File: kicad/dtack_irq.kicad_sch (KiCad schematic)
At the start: 18 parts, among them J10 Free pin, J11 Free Pins, J12 Free pins, J13 Free pins, J14 Free pin, J15 Free pin, J9 Free pin, U16 GAL22V10, U17 GAL22V10

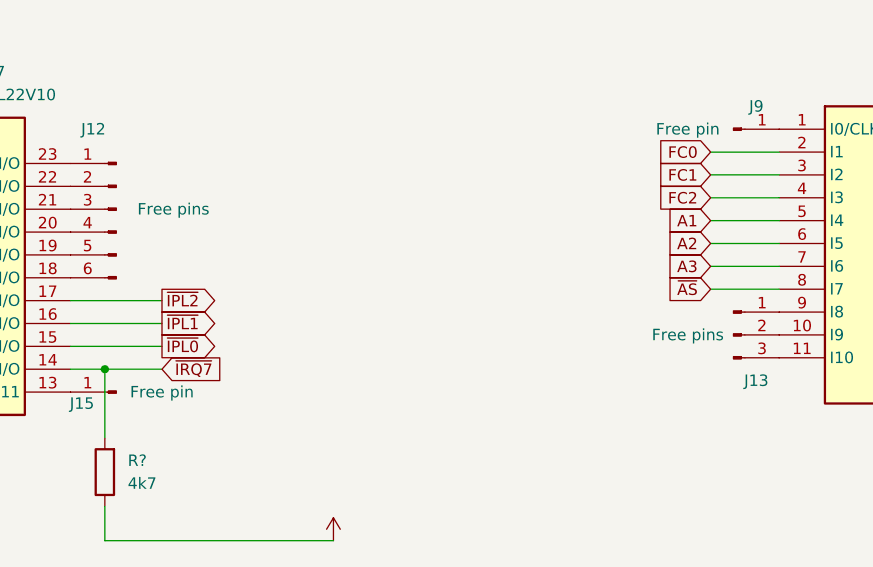
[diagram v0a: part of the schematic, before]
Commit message: fiddlign with placement
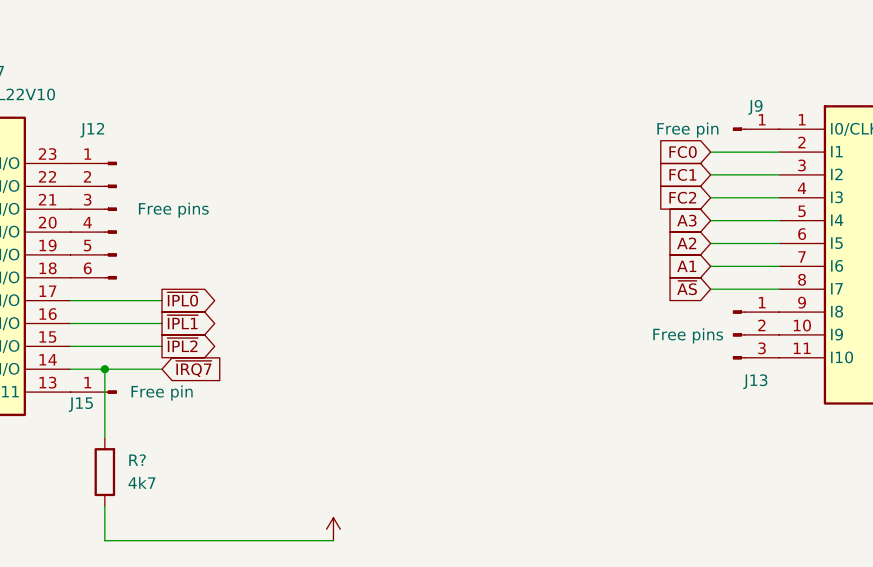
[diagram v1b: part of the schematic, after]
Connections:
- net A1: now also U16.7 (I6); no longer U16.5 (I4)
- net A3: now also U16.5 (I4); no longer U16.7 (I6)
- net ~{IPL0}: now also U17.17 (I/O); no longer U17.15 (I/O)
- net ~{IPL2}: now also U17.15 (I/O); no longer U17.17 (I/O)
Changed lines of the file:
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@@
     (effects (font (size 1.27 1.27)) (justify left bottom))
   )
-  (global_label "~{IPL2}" (shape output) (at 119.38 68.58 0) (fields_autoplaced)
+  (global_label "~{IPL2}" (shape output) (at 119.38 73.66 0) (fields_autoplaced)
     (effects (font (size 1.27 1.27)) (justify left))
-    (property "Intersheetrefs" "${INTERSHEET_REFS}" (at 126.3982 68.58 0)
+    (property "Intersheetrefs" "${INTERSHEET_REFS}" (at 126.3982 73.66 0)
       (effects (font (size 1.27 1.27)) (justify left) hide)
     )
@@
     )
   )
-  (global_label "A3" (shape input) (at 180.34 64.77 180) (fields_autoplaced)
+  (global_label "A3" (shape input) (at 180.34 59.69 180) (fields_autoplaced)
     (effects (font (size 1.27 1.27)) (justify right))
-    (property "Intersheetrefs" "${INTERSHEET_REFS}" (at 175.1361 64.77 0)
+    (property "Intersheetrefs" "${INTERSHEET_REFS}" (at 175.1361 59.69 0)
       (effects (font (size 1.27 1.27)) (justify right) hide)
     )
@@
     )
   )
-  (global_label "A1" (shape input) (at 180.34 59.69 180) (fields_autoplaced)
+  (global_label "A1" (shape input) (at 180.34 64.77 180) (fields_autoplaced)
     (effects (font (size 1.27 1.27)) (justify right))
-    (property "Intersheetrefs" "${INTERSHEET_REFS}" (at 175.1361 59.69 0)
+    (property "Intersheetrefs" "${INTERSHEET_REFS}" (at 175.1361 64.77 0)
       (effects (font (size 1.27 1.27)) (justify right) hide)
     )
@@
     )
   )
-  (global_label "~{IPL0}" (shape output) (at 119.38 73.66 0) (fields_autoplaced)
+  (global_label "~{IPL0}" (shape output) (at 119.38 68.58 0) (fields_autoplaced)
     (effects (font (size 1.27 1.27)) (justify left))
-    (property "Intersheetrefs" "${INTERSHEET_REFS}" (at 126.3982 73.66 0)
+    (property "Intersheetrefs" "${INTERSHEET_REFS}" (at 126.3982 68.58 0)
       (effects (font (size 1.27 1.27)) (justify left) hide)
     )
